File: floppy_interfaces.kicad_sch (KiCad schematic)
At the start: 24 parts, among them J13 Conn_01x04_Male, J14 Conn_02x17_Odd_Even, J16 Conn_01x04_Male, J6 SDF-60J for IEC 1541 serial p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, U1 74LS373, U2 74LVC374, U22 74LS06N, U3 74LVC374, U4 74LS373

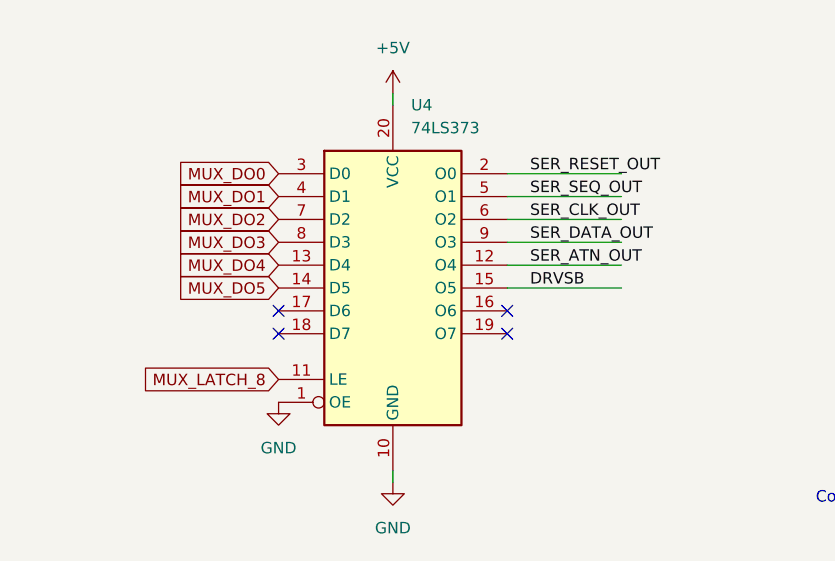
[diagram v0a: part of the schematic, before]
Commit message: route u4
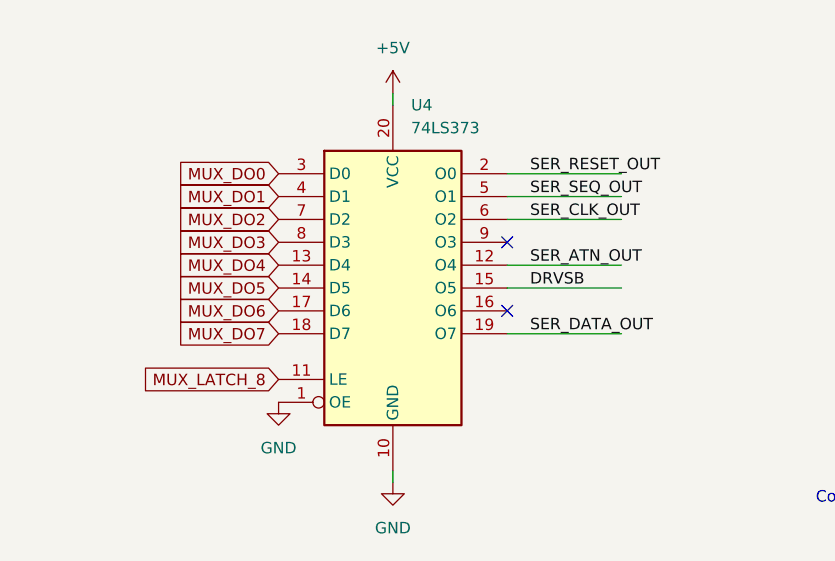
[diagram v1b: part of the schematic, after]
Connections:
- net MUX_DO6: now also U4.17 (D6)
- net MUX_DO7: now also U4.18 (D7)
- net SER_DATA_OUT: now also U4.19 (O7); no longer U4.9 (O3)
- no-connect marks 18 -> 16
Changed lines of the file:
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@@
   (no_connect (at 69.85 166.37))
   (no_connect (at 234.95 39.37))
-  (no_connect (at 156.21 171.45))
+  (no_connect (at 156.21 161.29))
   (no_connect (at 69.85 102.87))
-  (no_connect (at 130.81 168.91))
   (no_connect (at 44.45 105.41))
   (no_connect (at 44.45 171.45))
@@
   (no_connect (at 44.45 102.87))
   (no_connect (at 44.45 107.95))
-  (no_connect (at 130.81 171.45))
   (no_connect (at 234.95 41.91))
   (no_connect (at 69.85 107.95))
@@
     (stroke (width 0) (type default) (color 0 0 0 0))
   )
-  (wire (pts (xy 156.21 161.29) (xy 168.91 161.29))
+  (wire (pts (xy 156.21 171.45) (xy 168.91 171.45))
     (stroke (width 0) (type default) (color 0 0 0 0))
   )
@@
     (effects (font (size 1.27 1.27)) (justify left bottom))
   )
-  (label "SER_DATA_OUT" (at 158.75 161.29 0)
+  (label "SER_DATA_OUT" (at 158.75 171.45 0)
     (effects (font (size 1.27 1.27)) (justify left bottom))
   )
@@
     )
   )
+  (global_label "MUX_DO7" (shape input) (at 130.81 171.45 180) (fields_autoplaced)
+    (effects (font (size 1.27 1.27)) (justify right))
+    (property "Intersheet References" "${INTERSHEET_REFS}" (id 0) (at 119.6279 171.3706 0)
+      (effects (font (size 1.27 1.27)) (justify right) hide)
+    )
+  )
   (global_label "MUX_DO0" (shape input) (at 130.81 153.67 180) (fields_autoplaced)
     (effects (font (size 1.27 1.27)) (justify right))
@@
       (effects (font (size 1.27 1.27)) (justify right) hide)
     )
+  )
+  (global_label "MUX_DO6" (shape input) (at 130.81 168.91 180) (fields_autoplaced)
+    (effects (font (size 1.27 1.27)) (justify right))
+    (property "Intersheet References" "${INTERSHEET_REFS}" (id 0) (at 119.6279 168.8306 0)
+      (effects (font (size 1.27 1.27)) (justify right) hide)
+    )
